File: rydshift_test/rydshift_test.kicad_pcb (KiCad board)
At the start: 2 copper layers, 38.8 x 43.6 mm, 22 parts, among them IC1 PMA3-43-1W+, J1 RF INPUT, J2 RF OUTPUT, J3 DC IN, J4 TEST IN, J5 TEST OUT

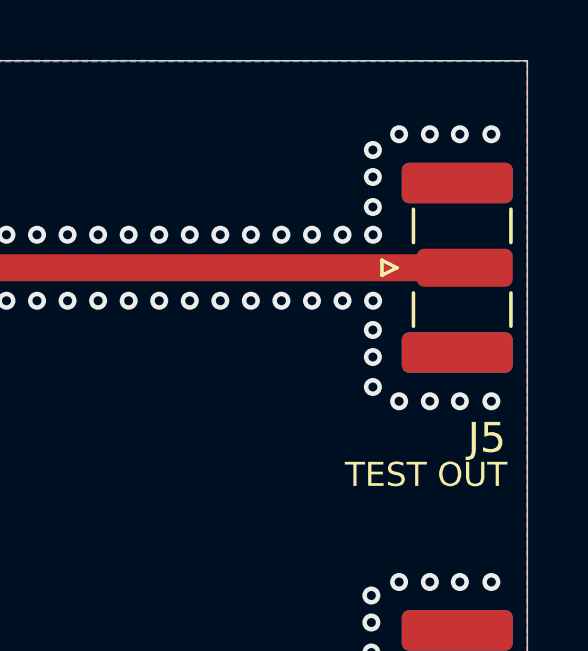
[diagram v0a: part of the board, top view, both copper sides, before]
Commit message: completed sch
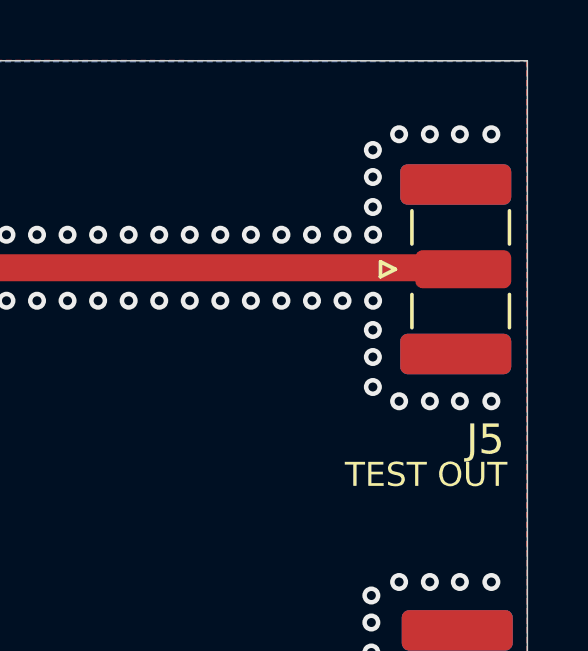
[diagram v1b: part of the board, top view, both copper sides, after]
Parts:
- moved J5 0.07 mm to (168.1, 62.9)
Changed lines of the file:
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@@
 	(footprint "Connector_Coaxial:SMA_Samtec_SMA-J-P-H-ST-EM1_EdgeMount"
 		(layer "F.Cu")
-		(at 168.1875 62.8)
+		(at 168.1375 62.85)
 		(descr "Connector SMA, 0Hz to 20GHz, 50Ohm, Edge Mount (http://suddendocs.samtec.com/prints/sma-j-p-x-st-em1-mkt.pdf)")
 		(tags "SMA Straight Samtec Edge Mount")
